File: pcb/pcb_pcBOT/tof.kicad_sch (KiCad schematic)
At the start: 5 parts, among them J501 vl053l0x

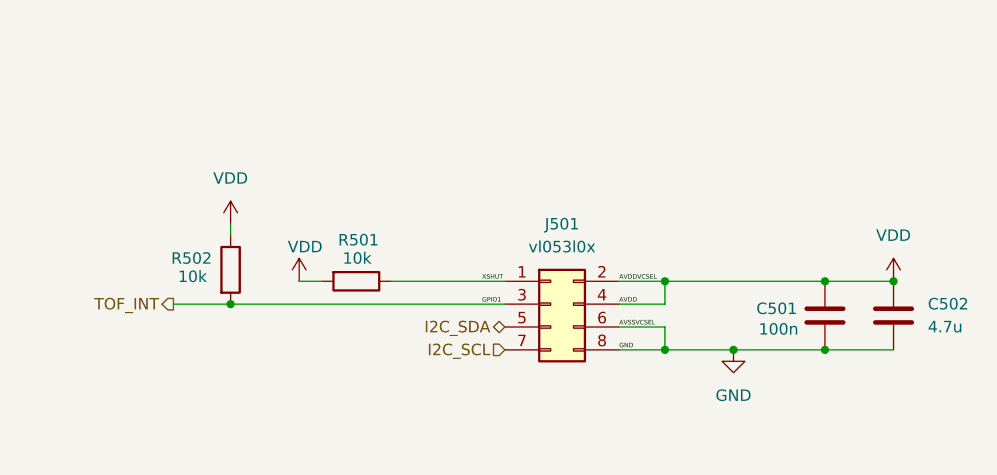
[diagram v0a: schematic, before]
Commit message: Revert "Ajout empreintes (incomplet) + test erc correct"
This reverts commit 267ed5519d67c336b99c9c80b0ac2067182b82a3.
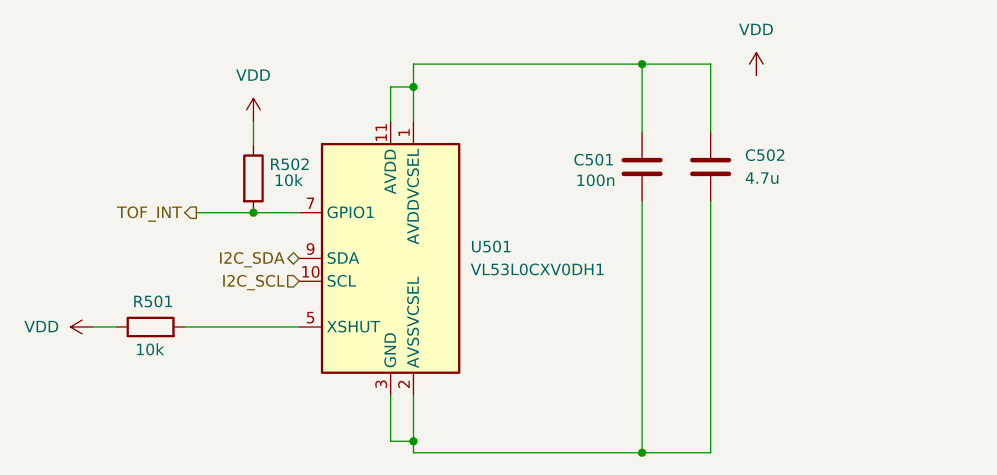
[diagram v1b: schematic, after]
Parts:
- removed J501: vl053l0x, symbol Connector_Generic:Conn_02x04_Odd_Even
- added U501: VL53L0CXV0DH1, Sensor_Distance:ST_VL53L1x, symbol Sensor_Distance:VL53L0CXV0DH1
- C501, C502: footprint Capacitor_SMD:C_0805_2012Metric_Pad1.18x1.45mm_HandSolder -> (none)
- R501, R502: footprint Resistor_SMD:R_0805_2012Metric_Pad1.20x1.40mm_HandSolder -> (none)
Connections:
- net XSHUT is gone; now on net VDD: R501.1
- net I2C_SCL: now also U501.10 (SCL)
- net I2C_SDA: now also U501.9 (SDA)
- net TOF_INT: now also U501.7 (GPIO1)
- net VDD: no longer C501.1, C502.1, R501.2
- net GND: no longer names the net of C501.2, C502.2
- net GND: now also U501.12 (GND), U501.2 (AVSSVCSEL), U501.3 (GND), U501.4 (GND), U501.6 (GND)
- new net: C501.1, C502.1, U501.1 (AVDDVCSEL), U501.11 (AVDD)
- new net: R501.2, U501.5 (XSHUT)
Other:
- moved on the sheet: C501, C502, R501, R502
